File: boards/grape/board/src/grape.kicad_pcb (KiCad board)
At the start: 4 copper layers, 84 x 64 mm, 136 parts, among them J1 USB-C USB2 Device, J2 GPIO 0-27, J3 GPIO 28-55, J4 JTAG, Q1 BSS138, SW1 IMAGE[1:0], SW2 COLD RESET, SW3 PROGRAM, U1 XC7A35T-1FTG256C, U2 TPS62A02DRL, U3 TPS62A02DRL, U4 TPS62A02DRL, U5 W25Q128JVSIQ, U6 USBLC6-2SC6, U7 TPS22917DBV, X1 ASE-48.000MHz

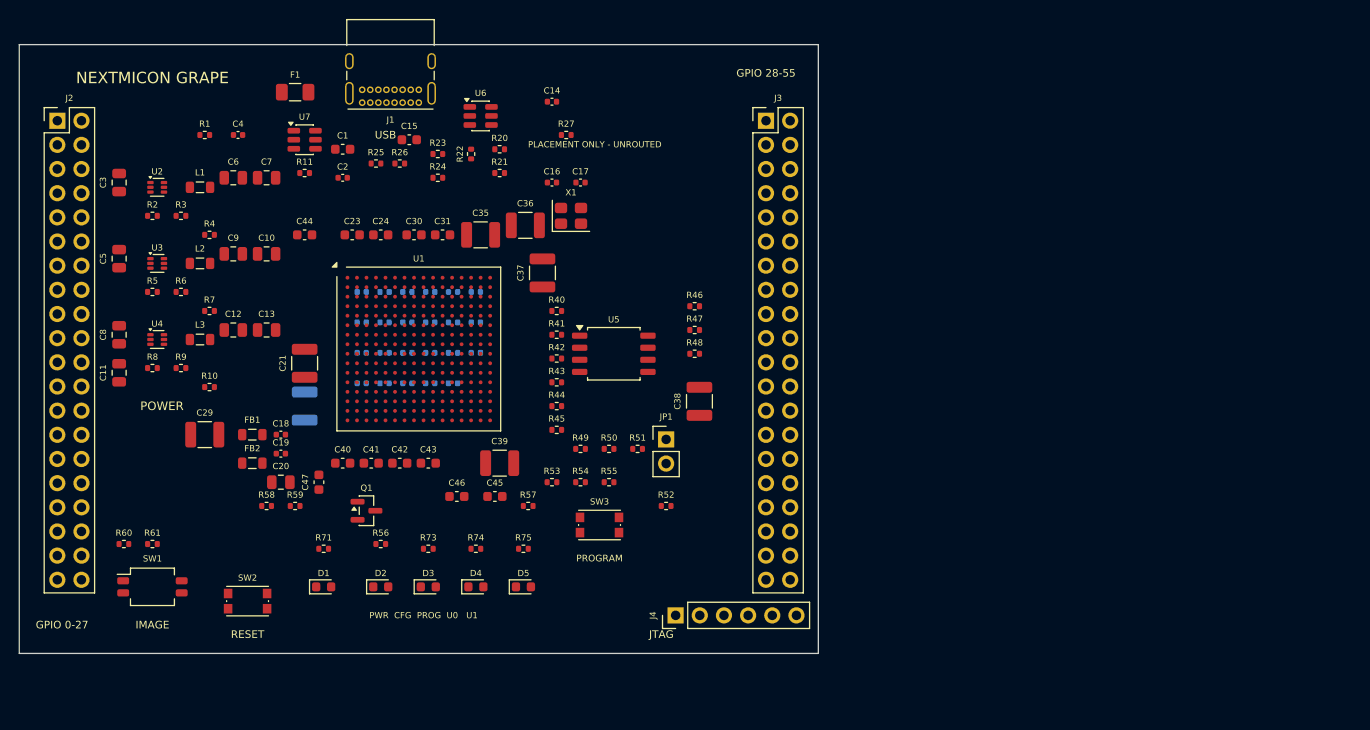
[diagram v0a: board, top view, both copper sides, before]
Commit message: wip
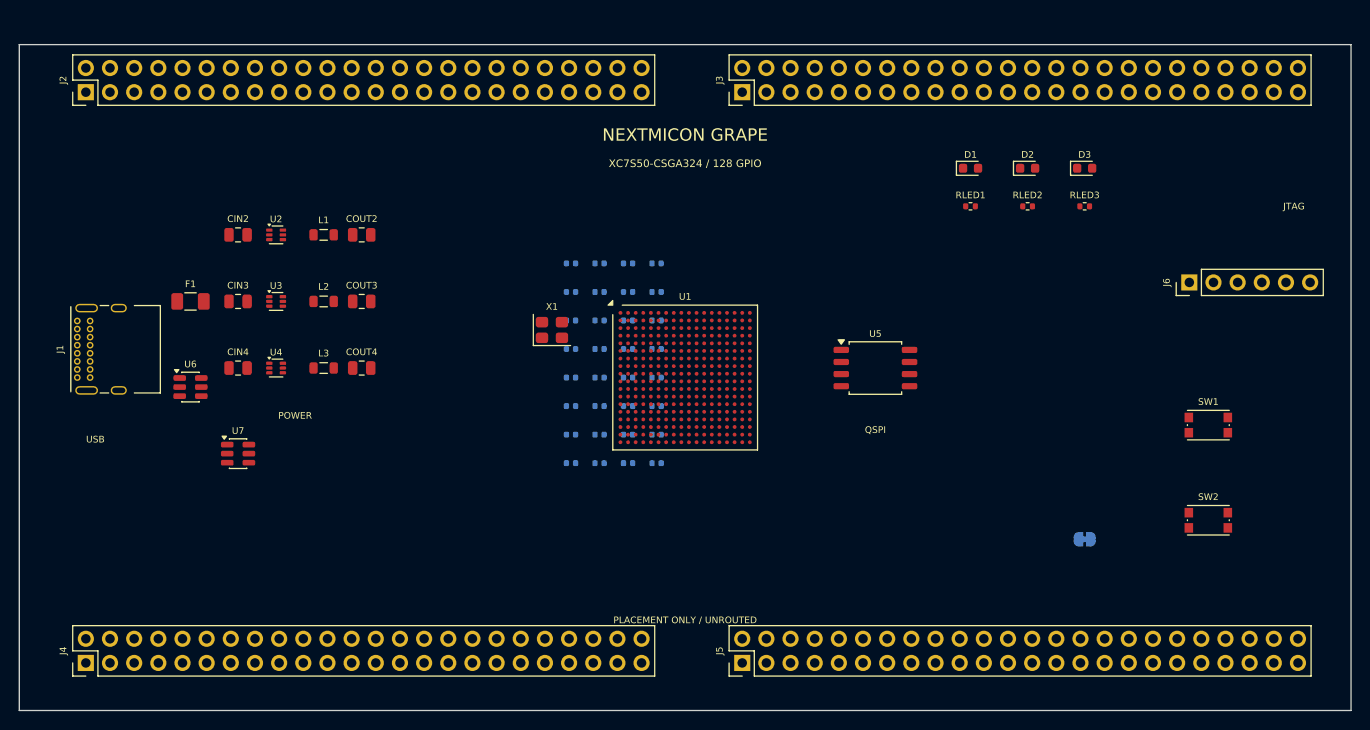
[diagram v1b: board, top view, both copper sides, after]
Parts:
- removed C1, C15: 1uF, Capacitor_SMD:C_0603_1608Metric
- removed C10, C12, C13, C6, C7, C9: 22uF, Capacitor_SMD:C_0805_2012Metric
- removed C11, C3, C5, C8: 10uF, Capacitor_SMD:C_0805_2012Metric
- removed C14: 4.7nF, Capacitor_SMD:C_0402_1005Metric
- removed C16, C17, C18, C4: 100nF, Capacitor_SMD:C_0402_1005Metric
- removed C19: 470nF, Capacitor_SMD:C_0402_1005Metric
- removed C2: 4.7nF TUNE, Capacitor_SMD:C_0402_1005Metric
- removed C52, C53, C54, C55, C56, C57, C58, C59, C60, C61, C62, C63: 0.47uF, Capacitor_SMD:C_0402_1005Metric
- removed D4: 4 LED, LED_SMD:LED_0603_1608Metric
- removed D5: 5 LED, LED_SMD:LED_0603_1608Metric
- removed FB1, FB2: 600R@100MHz, Inductor_SMD:L_0805_2012Metric
- removed Q1: BSS138, Package_TO_SOT_SMD:SOT-23
- removed R1, R10, R4, R7: 100k, Resistor_SMD:R_0402_1005Metric
- removed R11, R49, R53, R54, R55, R56, R71, R73, R74, R75: 1k, Resistor_SMD:R_0402_1005Metric
- removed R2: 66.5k 1%, Resistor_SMD:R_0402_1005Metric
- removed R20, R21, R40, R41, R42, R43, R44, R45: 22R TUNE, Resistor_SMD:R_0402_1005Metric
- removed R22: 1.5k, Resistor_SMD:R_0402_1005Metric
- removed R23, R24: 5.1k, Resistor_SMD:R_0402_1005Metric
- removed R25: 82k, Resistor_SMD:R_0402_1005Metric
- removed R26: 68k, Resistor_SMD:R_0402_1005Metric
- removed R27: 1M, Resistor_SMD:R_0402_1005Metric
- removed R3, R5, R8: 100k 1%, Resistor_SMD:R_0402_1005Metric
- removed R46: 2.4k, Resistor_SMD:R_0402_1005Metric
- removed R47, R48, R50, R51, R52: 4.7k, Resistor_SMD:R_0402_1005Metric
- removed R57, R58, R59: 0R, Resistor_SMD:R_0402_1005Metric
- removed R6: 49.9k 1%, Resistor_SMD:R_0402_1005Metric
- removed R60, R61: 10k, Resistor_SMD:R_0402_1005Metric
- removed R9: 22.1k 1%, Resistor_SMD:R_0402_1005Metric
- removed SW3: PROGRAM, Button_Switch_SMD:SW_Push_1P1T_NO_CK_KMR2
- added CIN2: 10uF, Capacitor_SMD:C_0805_2012Metric, F.Cu at (43.0, 40.0)
- added CIN3: 10uF, Capacitor_SMD:C_0805_2012Metric, F.Cu at (43.0, 47.0)
- added CIN4: 10uF, Capacitor_SMD:C_0805_2012Metric, F.Cu at (43.0, 54.0)
- added COUT2: 22uF, Capacitor_SMD:C_0805_2012Metric, F.Cu at (56.0, 40.0)
- added COUT3: 22uF, Capacitor_SMD:C_0805_2012Metric, F.Cu at (56.0, 47.0)
- added COUT4: 22uF, Capacitor_SMD:C_0805_2012Metric, F.Cu at (56.0, 54.0)
- added J5: GPIO 97-128, Connector_PinHeader_2.54mm:PinHeader_2x24_P2.54mm_Vertical, F.Cu at (96.0, 85.0)
- added J6: JTAG, Connector_PinHeader_2.54mm:PinHeader_1x06_P2.54mm_Vertical, F.Cu at (143.0, 45.0)
- added RLED1: 1k, Resistor_SMD:R_0402_1005Metric, F.Cu at (120.0, 37.0)
- added RLED2: 1k, Resistor_SMD:R_0402_1005Metric, F.Cu at (126.0, 37.0)
- added RLED3: 1k, Resistor_SMD:R_0402_1005Metric, F.Cu at (132.0, 37.0)
- C20: value 10uF -> 0.47uF; footprint Capacitor_SMD:C_0805_2012Metric -> Capacitor_SMD:C_0402_1005Metric; moved to B.Cu
- C21: value 100uF -> 0.47uF; footprint Capacitor_SMD:C_1210_3225Metric -> Capacitor_SMD:C_0402_1005Metric; moved to B.Cu
- C22: value 47uF -> 0.47uF; footprint Capacitor_SMD:C_1210_3225Metric -> Capacitor_SMD:C_0402_1005Metric
- C23, C24, C30, C31, C40, C41, C42, C43, C44, C45, C46, C47: value 4.7uF -> 0.47uF; footprint Capacitor_SMD:C_0603_1608Metric -> Capacitor_SMD:C_0402_1005Metric; moved to B.Cu
- C29, C35, C36, C37, C38, C39: value 47uF -> 0.47uF; footprint Capacitor_SMD:C_1210_3225Metric -> Capacitor_SMD:C_0402_1005Metric; moved to B.Cu
- D1: value 1 LED -> STATUS LED
- D2: value CFG DONE -> STATUS LED
- D3: value 3 LED -> STATUS LED
- F1: value 1.1A hold -> 1.1A HOLD
- J2: value GPIO 0-27 -> GPIO 1-32; footprint Connector_PinHeader_2.54mm:PinHeader_2x20_P2.54mm_Vertical -> Connector_PinHeader_2.54mm:PinHeader_2x24_P2.54mm_Vertical
- J3: value GPIO 28-55 -> GPIO 33-64; footprint Connector_PinHeader_2.54mm:PinHeader_2x20_P2.54mm_Vertical -> Connector_PinHeader_2.54mm:PinHeader_2x24_P2.54mm_Vertical
- J4: value JTAG -> GPIO 65-96; footprint Connector_PinHeader_2.54mm:PinHeader_1x06_P2.54mm_Vertical -> Connector_PinHeader_2.54mm:PinHeader_2x24_P2.54mm_Vertical
- JP1: value GOLDEN_LOCK (fit for x1) -> DEFAULT_USER; footprint Connector_PinHeader_2.54mm:PinHeader_1x02_P2.54mm_Vertical -> Jumper:SolderJumper-2_P1.3mm_Bridged_RoundedPad1.0x1.5mm; moved to B.Cu
- L1, L2, L3: value 1uH >=2.5A -> 1uH
- SW1: value IMAGE[1:0] -> PROGRAM; footprint Button_Switch_SMD:SW_DIP_SPSTx02_Slide_Omron_A6H-2101_W6.15mm_P1.27mm -> Button_Switch_SMD:SW_Push_1P1T_NO_CK_KMR2
- SW2: value COLD RESET -> USER
- U1: value XC7A35T-1FTG256C -> XC7S50-1CSGA324C; footprint Package_BGA:Xilinx_FTG256 -> Package_BGA:Xilinx_CSGA324
- X1: value ASE-48.000MHz -> 100MHz XO
- moved SW1 112.3 mm to (145.0, 60.0)
- moved SW2 101.4 mm to (145.0, 70.0)
- moved D3 81.8 mm to (132.0, 33.0)
- moved D1 81.0 mm to (120.0, 33.0)
- moved D2 81.0 mm to (126.0, 33.0)
- moved J4 62.2 mm to (27.0, 85.0)
- moved J1 46.1 mm to (26.1, 55.0), turned to 90 degrees
- moved JP1 45.2 mm to (132.0, 72.0)
- moved C29 43.2 mm to (81.0, 49.0)
- moved U6 41.7 mm to (38.0, 56.0)
- moved C20 38.2 mm to (78.0, 43.0)
- moved C22 37.2 mm to (84.0, 43.0), turned to 0 degrees
- moved C47 35.9 mm to (87.0, 61.0), turned to 0 degrees
- moved C44 35.0 mm to (78.0, 61.0)
- moved U7 33.7 mm to (43.0, 63.0)
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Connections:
- C20 pad 1: /+1V8A -> (no net)
- C20 pad 2: /AGND -> (no net)
- C21 pad 1: /+1V0 -> (no net)
- C21 pad 2: /GND -> (no net)
- C22 pad 1: /+1V0 -> (no net)
- C22 pad 2: /GND -> (no net)
- C23 pad 1: /+1V0 -> (no net)
- C23 pad 2: /GND -> (no net)
- C24 pad 1: /+1V0 -> (no net)
- C24 pad 2: /GND -> (no net)
- C25 pad 1: /+1V0 -> (no net)
- C25 pad 2: /GND -> (no net)
- C26 pad 1: /+1V0 -> (no net)
- C26 pad 2: /GND -> (no net)
- C27 pad 1: /+1V0 -> (no net)
- C27 pad 2: /GND -> (no net)
- C28 pad 1: /+1V0 -> (no net)
- C28 pad 2: /GND -> (no net)
- C29 pad 1: /+1V8 -> (no net)
- C29 pad 2: /GND -> (no net)
- C30 pad 1: /+1V8 -> (no net)
- C30 pad 2: /GND -> (no net)
- C31 pad 1: /+1V8 -> (no net)
- C31 pad 2: /GND -> (no net)
- C32 pad 1: /+1V8 -> (no net)
- C32 pad 2: /GND -> (no net)
- C33 pad 1: /+1V8 -> (no net)
- C33 pad 2: /GND -> (no net)
- C34 pad 1: /+1V8 -> (no net)
- C34 pad 2: /GND -> (no net)
- C35 pad 1: /+3V3 -> (no net)
- C35 pad 2: /GND -> (no net)
- C36 pad 1: /+3V3 -> (no net)
- C36 pad 2: /GND -> (no net)
- C37 pad 1: /+3V3 -> (no net)
- C37 pad 2: /GND -> (no net)
- C38 pad 1: /+3V3 -> (no net)
- C38 pad 2: /GND -> (no net)
- C39 pad 1: /+3V3 -> (no net)
- C39 pad 2: /GND -> (no net)
- C40 pad 1: /+3V3 -> (no net)
- C40 pad 2: /GND -> (no net)
- C41 pad 1: /+3V3 -> (no net)
- C41 pad 2: /GND -> (no net)
- C42 pad 1: /+3V3 -> (no net)
- C42 pad 2: /GND -> (no net)
- C43 pad 1: /+3V3 -> (no net)
- C43 pad 2: /GND -> (no net)
- C44 pad 1: /+3V3 -> (no net)
- C44 pad 2: /GND -> (no net)
- C45 pad 1: /+3V3 -> (no net)
- C45 pad 2: /GND -> (no net)
- C46 pad 1: /+3V3 -> (no net)
- C46 pad 2: /GND -> (no net)
- C47 pad 1: /+3V3 -> (no net)
- C47 pad 2: /GND -> (no net)
- C48 pad 1: /+3V3 -> (no net)
- C48 pad 2: /GND -> (no net)
- C49 pad 1: /+3V3 -> (no net)
- C49 pad 2: /GND -> (no net)
- C50 pad 1: /+3V3 -> (no net)
- C50 pad 2: /GND -> (no net)
- C51 pad 1: /+3V3 -> (no net)
- C51 pad 2: /GND -> (no net)
- D1 pad 1: /GND -> (no net)
- D1 pad 2: /D1_A -> (no net)
- D2 pad 1: /DONE_LED_K -> (no net)
- D2 pad 2: /DONE_LED_A -> (no net)
- D3 pad 1: /GND -> (no net)
- D3 pad 2: /D3_A -> (no net)
- F1 pad 1: /VBUS -> (no net)
- F1 pad 2: /VBUS_FUSED -> (no net)
- J1 pad A1: /GND -> (no net)
- J1 pad A12: /GND -> (no net)
- J1 pad A4: /VBUS -> (no net)
- J1 pad A5: /USB_CC1 -> (no net)
- J1 pad A6: /USB_DP_CONN -> (no net)
- J1 pad A7: /USB_DM_CONN -> (no net)
- J1 pad A8: unconnected-(J1-SBU1-PadA8) -> (no net)
- J1 pad A9: /VBUS -> (no net)
- J1 pad B1: /GND -> (no net)
- J1 pad B12: /GND -> (no net)
- J1 pad B4: /VBUS -> (no net)
- J1 pad B5: /USB_CC2 -> (no net)
- J1 pad B6: /USB_DP_CONN -> (no net)
- J1 pad B7: /USB_DM_CONN -> (no net)
- J1 pad B8: unconnected-(J1-SBU2-PadB8) -> (no net)
- J1 pad B9: /VBUS -> (no net)
- J1 pad SH: /USB_SHIELD -> (no net)
- J2 pad 1: /+3V3 -> (no net)
- J2 pad 10: /GPIO_07 -> (no net)
- J2 pad 11: /GND -> (no net)
- J2 pad 12: /GND -> (no net)
- J2 pad 13: /GPIO_08 -> (no net)
- J2 pad 14: /GPIO_09 -> (no net)
- J2 pad 15: /GPIO_10 -> (no net)
- J2 pad 16: /GPIO_11 -> (no net)
- J2 pad 17: /GPIO_12 -> (no net)
- J2 pad 18: /GPIO_13 -> (no net)
- J2 pad 19: /GPIO_14 -> (no net)
- J2 pad 2: /+5V -> (no net)
- J2 pad 20: /GPIO_15 -> (no net)
- J2 pad 21: /+3V3 -> (no net)
- J2 pad 22: /GND -> (no net)
- J2 pad 23: /GPIO_16 -> (no net)
- J2 pad 24: /GPIO_17 -> (no net)
- J2 pad 25: /GPIO_18 -> (no net)
- J2 pad 26: /GPIO_19 -> (no net)
- J2 pad 27: /GPIO_20 -> (no net)
- J2 pad 28: /GPIO_21 -> (no net)
- J2 pad 29: /GPIO_22 -> (no net)
- J2 pad 3: /GPIO_00 -> (no net)
- J2 pad 30: /GPIO_23 -> (no net)
- J2 pad 31: /GND -> (no net)
- J2 pad 32: /GND -> (no net)
- J2 pad 33: /GPIO_24 -> (no net)
- J2 pad 34: /GPIO_25 -> (no net)
- J2 pad 35: /GPIO_26 -> (no net)
- J2 pad 36: /GPIO_27 -> (no net)
- J2 pad 37: /GND -> (no net)
- J2 pad 38: /GND -> (no net)
- J2 pad 39: /+3V3 -> (no net)
- J2 pad 4: /GPIO_01 -> (no net)
- J2 pad 40: /+5V -> (no net)
- J2 pad 5: /GPIO_02 -> (no net)
- J2 pad 6: /GPIO_03 -> (no net)
- J2 pad 7: /GPIO_04 -> (no net)
- J2 pad 8: /GPIO_05 -> (no net)
- J2 pad 9: /GPIO_06 -> (no net)
- J3 pad 1: /+3V3 -> (no net)
- J3 pad 10: /GPIO_35 -> (no net)
- J3 pad 11: /GND -> (no net)
- J3 pad 12: /GND -> (no net)
- J3 pad 13: /GPIO_36 -> (no net)
- J3 pad 14: /GPIO_37 -> (no net)
- J3 pad 15: /GPIO_38 -> (no net)
- J3 pad 16: /GPIO_39 -> (no net)
- J3 pad 17: /GPIO_40 -> (no net)
- J3 pad 18: /GPIO_41 -> (no net)
- J3 pad 19: /GPIO_42 -> (no net)
- J3 pad 2: /+5V -> (no net)
- J3 pad 20: /GPIO_43 -> (no net)
- J3 pad 21: /+3V3 -> (no net)
- J3 pad 22: /GND -> (no net)
- J3 pad 23: /GPIO_44 -> (no net)
- J3 pad 24: /GPIO_45 -> (no net)
- J3 pad 25: /GPIO_46 -> (no net)
- J3 pad 26: /GPIO_47 -> (no net)
- J3 pad 27: /GPIO_48 -> (no net)
- J3 pad 28: /GPIO_49 -> (no net)
- J3 pad 29: /GPIO_50 -> (no net)
- J3 pad 3: /GPIO_28 -> (no net)
- J3 pad 30: /GPIO_51 -> (no net)
- J3 pad 31: /GND -> (no net)
- J3 pad 32: /GND -> (no net)
- J3 pad 33: /GPIO_52 -> (no net)
- J3 pad 34: /GPIO_53 -> (no net)
- J3 pad 35: /GPIO_54 -> (no net)
- J3 pad 36: /GPIO_55 -> (no net)
- J3 pad 37: /GND -> (no net)
- J3 pad 38: /GND -> (no net)
- J3 pad 39: /+3V3 -> (no net)
- J3 pad 4: /GPIO_29 -> (no net)
- J3 pad 40: /+5V -> (no net)
- J3 pad 5: /GPIO_30 -> (no net)
- J3 pad 6: /GPIO_31 -> (no net)
- J3 pad 7: /GPIO_32 -> (no net)
- J3 pad 8: /GPIO_33 -> (no net)
- J3 pad 9: /GPIO_34 -> (no net)
- J4 pad 1: /+3V3 -> (no net)
- J4 pad 2: /GND -> (no net)
- J4 pad 3: /JTAG_TCK -> (no net)
- J4 pad 4: /JTAG_TMS -> (no net)
- J4 pad 5: /JTAG_TDI -> (no net)
- J4 pad 6: /JTAG_TDO -> (no net)
- JP1 pad 1: /QSPI_IO2 -> (no net)
- JP1 pad 2: /GND -> (no net)
- L1 pad 1: /+1V0_SW -> (no net)
- L1 pad 2: /+1V0 -> (no net)
- L2 pad 1: /+1V8_SW -> (no net)
- L2 pad 2: /+1V8 -> (no net)
- L3 pad 1: /+3V3_SW -> (no net)
- L3 pad 2: /+3V3 -> (no net)
- SW1 pad 1: /IMAGE0 -> (no net)
- SW1 pad 2: /IMAGE1 -> (no net)
- SW2 pad 1: /PWR_EN -> (no net)
- SW2 pad 2: /GND -> (no net)
- U1 pad A1: /GND -> (no net)
- U1 pad A10: unconnected-(U1A-IO_L3N_T0_DQS_AD1N_15-PadA10) -> (no net)
- U1 pad A11: /GND -> (no net)
- U1 pad A12: unconnected-(U1A-IO_L5N_T0_AD9N_15-PadA12) -> (no net)
- U1 pad A13: unconnected-(U1A-IO_L7P_T1_AD2P_15-PadA13) -> (no net)
- U1 pad A14: unconnected-(U1A-IO_L7N_T1_AD2N_15-PadA14) -> (no net)
- U1 pad A15: unconnected-(U1A-IO_L9N_T1_DQS_AD3N_15-PadA15) -> (no net)
- U1 pad A16: /+3V3 -> (no net)
- U1 pad A2: /USER_LED1 -> (no net)
- U1 pad A3: /IMAGE0 -> (no net)
- U1 pad A4: /PROG_LED -> (no net)
- U1 pad A5: /USER_LED0 -> (no net)
- U1 pad A6: /+3V3 -> (no net)
- U1 pad A7: /VBUS_SENSE -> (no net)
- U1 pad A8: unconnected-(U1A-IO_L2P_T0_AD8P_15-PadA8) -> (no net)
- U1 pad A9: unconnected-(U1A-IO_L2N_T0_AD8N_15-PadA9) -> (no net)
- U1 pad B1: /GPIO_00 -> (no net)
- U1 pad B10: unconnected-(U1A-IO_L4P_T0_15-PadB10) -> (no net)
- U1 pad B11: unconnected-(U1A-IO_L4N_T0_15-PadB11) -> (no net)
- U1 pad B12: unconnected-(U1A-IO_L5P_T0_AD9P_15-PadB12) -> (no net)
- U1 pad B13: /+3V3 -> (no net)
- U1 pad B14: unconnected-(U1A-IO_L8N_T1_AD10N_15-PadB14) -> (no net)
- U1 pad B15: unconnected-(U1A-IO_L9P_T1_DQS_AD3P_15-PadB15) -> (no net)
- U1 pad B16: unconnected-(U1A-IO_L10N_T1_AD11N_15-PadB16) -> (no net)
- U1 pad B2: /GPIO_01 -> (no net)
- U1 pad B3: /+3V3 -> (no net)
- U1 pad B4: /IMAGE1 -> (no net)
- U1 pad B5: /USB_DM -> (no net)
- U1 pad B6: /USB_DP -> (no net)
- U1 pad B7: /USB_PULLUP -> (no net)
- U1 pad B8: /GND -> (no net)
- U1 pad B9: unconnected-(U1A-IO_L3P_T0_DQS_AD1P_15-PadB9) -> (no net)
- U1 pad C1: /GPIO_02 -> (no net)
- U1 pad C10: /+3V3 -> (no net)
- U1 pad C11: unconnected-(U1A-IO_L11P_T1_SRCC_15-PadC11) -> (no net)
- U1 pad C12: unconnected-(U1A-IO_L11N_T1_SRCC_15-PadC12) -> (no net)
- U1 pad C13: unconnected-(U1A-IO_L12N_T1_MRCC_15-PadC13) -> (no net)
- U1 pad C14: unconnected-(U1A-IO_L8P_T1_AD10P_15-PadC14) -> (no net)
- U1 pad C15: /GND -> (no net)
- U1 pad C16: unconnected-(U1A-IO_L10P_T1_AD11P_15-PadC16) -> (no net)
- U1 pad C2: /GPIO_03 -> (no net)
- U1 pad C3: /GPIO_04 -> (no net)
- U1 pad C4: /GPIO_05 -> (no net)
- U1 pad C5: /GND -> (no net)
- U1 pad C6: /GPIO_06 -> (no net)
- U1 pad C7: /GPIO_07 -> (no net)
- U1 pad C8: unconnected-(U1A-IO_L1P_T0_AD0P_15-PadC8) -> (no net)
- U1 pad C9: unconnected-(U1A-IO_L1N_T0_AD0N_15-PadC9) -> (no net)
- U1 pad D1: /GPIO_08 -> (no net)
- U1 pad D10: unconnected-(U1A-IO_0_15-PadD10) -> (no net)
- U1 pad D11: unconnected-(U1A-IO_L14N_T2_SRCC_15-PadD11) -> (no net)
- U1 pad D12: /GND -> (no net)
- U1 pad D13: unconnected-(U1A-IO_L12P_T1_MRCC_15-PadD13) -> (no net)
- U1 pad D14: unconnected-(U1A-IO_L15P_T2_DQS_15-PadD14) -> (no net)
- U1 pad D15: unconnected-(U1A-IO_L15N_T2_DQS_ADV_B_15-PadD15) -> (no net)
- U1 pad D16: unconnected-(U1A-IO_L17N_T2_A25_15-PadD16) -> (no net)
- U1 pad D2: /GND -> (no net)
- U1 pad D3: /GPIO_09 -> (no net)
- U1 pad D4: /GPIO_10 -> (no net)
- U1 pad D5: /GPIO_11 -> (no net)
- U1 pad D6: /GPIO_12 -> (no net)
- U1 pad D7: /+3V3 -> (no net)
- U1 pad D8: unconnected-(U1A-IO_L6P_T0_15-PadD8) -> (no net)
- U1 pad D9: unconnected-(U1A-IO_L6N_T0_VREF_15-PadD9) -> (no net)
- U1 pad E1: /GPIO_13 -> (no net)
- U1 pad E10: /+1V0 -> (no net)
- U1 pad E11: unconnected-(U1A-IO_L14P_T2_SRCC_15-PadE11) -> (no net)
- U1 pad E12: unconnected-(U1A-IO_L13P_T2_MRCC_15-PadE12) -> (no net)
- U1 pad E13: unconnected-(U1A-IO_L13N_T2_MRCC_15-PadE13) -> (no net)
- U1 pad E14: /+3V3 -> (no net)
- U1 pad E15: unconnected-(U1A-IO_L18N_T2_A23_15-PadE15) -> (no net)
- U1 pad E16: unconnected-(U1A-IO_L17P_T2_A26_15-PadE16) -> (no net)
- U1 pad E2: /GPIO_14 -> (no net)
- U1 pad E3: /CLK48 -> (no net)
- U1 pad E4: /+3V3 -> (no net)
- U1 pad E5: /GPIO_15 -> (no net)
- U1 pad E6: /GPIO_16 -> (no net)
- U1 pad E7: /CFGBVS_3V3 -> (no net)
- U1 pad E8: /QSPI_CCLK_FPGA -> (no net)
- U1 pad E9: /GND -> (no net)
- U1 pad F1: /+3V3 -> (no net)
- U1 pad F10: /GND -> (no net)
- U1 pad F11: /+1V0 -> (no net)
- U1 pad F12: unconnected-(U1A-IO_L16P_T2_A28_15-PadF12) -> (no net)
- U1 pad F13: unconnected-(U1A-IO_L16N_T2_A27_15-PadF13) -> (no net)
- U1 pad F14: unconnected-(U1A-IO_L21N_T3_DQS_A18_15-PadF14) -> (no net)
- U1 pad F15: unconnected-(U1A-IO_L18P_T2_A24_15-PadF15) -> (no net)
- U1 pad F16: /GND -> (no net)
- U1 pad F2: /GPIO_17 -> (no net)
- U1 pad F3: /GPIO_18 -> (no net)
- U1 pad F4: /GPIO_19 -> (no net)
- U1 pad F5: /GPIO_20 -> (no net)
- U1 pad F6: /GND -> (no net)
- U1 pad F7: /+1V0 -> (no net)
- U1 pad F8: /GND -> (no net)
- U1 pad F9: /+1V0 -> (no net)
- U1 pad G1: /GPIO_21 -> (no net)
- U1 pad G10: /+1V8 -> (no net)
- U1 pad G11: unconnected-(U1A-IO_25_15-PadG11) -> (no net)
- U1 pad G12: unconnected-(U1A-IO_L19N_T3_A21_VREF_15-PadG12) -> (no net)
- U1 pad G13: /GND -> (no net)
- U1 pad G14: unconnected-(U1A-IO_L21P_T3_DQS_15-PadG14) -> (no net)
- U1 pad G15: unconnected-(U1A-IO_L24N_T3_RS0_15-PadG15) -> (no net)
- U1 pad G16: unconnected-(U1A-IO_L22N_T3_A16_15-PadG16) -> (no net)
- U1 pad G2: /GPIO_22 -> (no net)
- U1 pad G3: /GND -> (no net)
- U1 pad G4: /GPIO_23 -> (no net)
- U1 pad G5: /GPIO_24 -> (no net)
- U1 pad G6: /+1V0 -> (no net)
- U1 pad G7: /AGND -> (no net)
- U1 pad G8: /+1V8A -> (no net)
- U1 pad G9: /GND -> (no net)
- U1 pad H1: /GPIO_25 -> (no net)
- U1 pad H10: /DONE -> (no net)
- U1 pad H11: unconnected-(U1A-IO_L19P_T3_A22_15-PadH11) -> (no net)
- U1 pad H12: unconnected-(U1A-IO_L20P_T3_A20_15-PadH12) -> (no net)
- U1 pad H13: unconnected-(U1A-IO_L20N_T3_A19_15-PadH13) -> (no net)
- U1 pad H14: unconnected-(U1A-IO_L24P_T3_RS1_15-PadH14) -> (no net)
- U1 pad H15: /+3V3 -> (no net)
- U1 pad H16: unconnected-(U1A-IO_L22P_T3_A17_15-PadH16) -> (no net)
- U1 pad H2: /GPIO_26 -> (no net)
- U1 pad H3: /GPIO_27 -> (no net)
- U1 pad H4: /GPIO_28 -> (no net)
- U1 pad H5: /GPIO_29 -> (no net)
- U1 pad H6: /GND -> (no net)
- U1 pad H7: /VREFN_AGND -> (no net)
- U1 pad H8: unconnected-(U1C-VP_0-PadH8) -> (no net)
- U1 pad H9: /+1V0 -> (no net)
- U1 pad J1: /GPIO_30 -> (no net)
- U1 pad J10: /+1V8 -> (no net)
- U1 pad J11: /GND -> (no net)
- U1 pad J12: /+3V3 -> (no net)
- U1 pad J13: /QSPI_IO0_FPGA -> (no net)
- U1 pad J14: /QSPI_IO1_FPGA -> (no net)
- U1 pad J15: unconnected-(U1A-IO_L23P_T3_FOE_B_15-PadJ15) -> (no net)
- U1 pad J16: unconnected-(U1A-IO_L23N_T3_FWE_B_15-PadJ16) -> (no net)
- U1 pad J2: /+3V3 -> (no net)
- U1 pad J3: /GPIO_31 -> (no net)
- U1 pad J4: /GPIO_32 -> (no net)
- U1 pad J5: /GPIO_33 -> (no net)
- U1 pad J6: /+1V0 -> (no net)
- U1 pad J7: unconnected-(U1C-VN_0-PadJ7) -> (no net)
- U1 pad J8: /VREFP_AGND -> (no net)
- U1 pad J9: /GND -> (no net)
- U1 pad K1: /GPIO_34 -> (no net)
- U1 pad K10: /INIT_B -> (no net)
- U1 pad K11: /+1V8 -> (no net)
- U1 pad K12: unconnected-(U1A-IO_0_14-PadK12) -> (no net)
- U1 pad K13: unconnected-(U1A-IO_L5P_T0_D06_14-PadK13) -> (no net)
- U1 pad K14: /GND -> (no net)
- U1 pad K15: /QSPI_IO2_FPGA -> (no net)
- U1 pad K16: /QSPI_IO3_FPGA -> (no net)
- U1 pad K2: /GPIO_35 -> (no net)
- U1 pad K3: /GPIO_36 -> (no net)
- U1 pad K4: /GND -> (no net)
- U1 pad K5: /GPIO_37 -> (no net)
- U1 pad K6: /GND -> (no net)
- U1 pad K7: unconnected-(U1C-DXN_0-PadK7) -> (no net)
- U1 pad K8: unconnected-(U1C-DXP_0-PadK8) -> (no net)
- U1 pad K9: /+1V0 -> (no net)
- U1 pad L1: /GND -> (no net)
- U1 pad L10: /+1V8 -> (no net)
- U1 pad L11: /GND -> (no net)
- U1 pad L12: /QSPI_CS_B_FPGA -> (no net)
- U1 pad L13: unconnected-(U1A-IO_L5N_T0_D07_14-PadL13) -> (no net)
- U1 pad L14: unconnected-(U1A-IO_L4P_T0_D04_14-PadL14) -> (no net)
- U1 pad L15: /PUDC_B -> (no net)
- U1 pad L16: /+3V3 -> (no net)
- U1 pad L2: /GPIO_38 -> (no net)
- U1 pad L3: /GPIO_39 -> (no net)
- U1 pad L4: /GPIO_40 -> (no net)
- U1 pad L5: /GPIO_41 -> (no net)
- U1 pad L6: /+3V3 -> (no net)
- U1 pad L7: /JTAG_TCK -> (no net)
- U1 pad L8: /+1V0 -> (no net)
- U1 pad L9: /PROGRAM_B -> (no net)
- U1 pad M1: /GPIO_42 -> (no net)
- U1 pad M10: /MODE_M1 -> (no net)
- U1 pad M11: /MODE_M2 -> (no net)
- U1 pad M12: unconnected-(U1A-IO_L6N_T0_D08_VREF_14-PadM12) -> (no net)
- U1 pad M13: /+3V3 -> (no net)
- U1 pad M14: unconnected-(U1A-IO_L4N_T0_D05_14-PadM14) -> (no net)
- U1 pad M15: unconnected-(U1A-IO_L3N_T0_DQS_EMCCLK_14-PadM15) -> (no net)
- U1 pad M16: unconnected-(U1A-IO_L7P_T1_D09_14-PadM16) -> (no net)
- U1 pad M2: /GPIO_43 -> (no net)
- U1 pad M3: /+3V3 -> (no net)
- U1 pad M4: /GPIO_44 -> (no net)
- U1 pad M5: /GPIO_45 -> (no net)
- U1 pad M6: unconnected-(U1A-IO_L19P_T3_A10_D26_14-PadM6) -> (no net)
- U1 pad M7: /JTAG_TMS -> (no net)
- U1 pad M8: /GND -> (no net)
- U1 pad M9: /MODE_M0 -> (no net)
- U1 pad N1: /GPIO_46 -> (no net)
- U1 pad N10: /+3V3 -> (no net)
- U1 pad N11: unconnected-(U1A-IO_L13P_T2_MRCC_14-PadN11) -> (no net)
- U1 pad N12: unconnected-(U1A-IO_L13N_T2_MRCC_14-PadN12) -> (no net)
- U1 pad N13: unconnected-(U1A-IO_L11P_T1_SRCC_14-PadN13) -> (no net)
- U1 pad N14: unconnected-(U1A-IO_L12P_T1_MRCC_14-PadN14) -> (no net)
- U1 pad N15: /GND -> (no net)
- U1 pad N16: unconnected-(U1A-IO_L7N_T1_D10_14-PadN16) -> (no net)
- U1 pad N2: /GPIO_47 -> (no net)
- U1 pad N3: /GPIO_48 -> (no net)
- U1 pad N4: /GPIO_49 -> (no net)
- U1 pad N5: /GND -> (no net)
- U1 pad N6: unconnected-(U1A-IO_L19N_T3_A09_D25_VREF_14-PadN6) -> (no net)
- U1 pad N7: /JTAG_TDI -> (no net)
- U1 pad N8: /JTAG_TDO -> (no net)
- U1 pad N9: unconnected-(U1A-IO_L18P_T2_A12_D28_14-PadN9) -> (no net)
- U1 pad P1: /GPIO_50 -> (no net)
- U1 pad P10: unconnected-(U1A-IO_L14P_T2_SRCC_14-PadP10) -> (no net)
- U1 pad P11: unconnected-(U1A-IO_L14N_T2_SRCC_14-PadP11) -> (no net)
- U1 pad P12: /GND -> (no net)
- U1 pad P13: unconnected-(U1A-IO_L11N_T1_SRCC_14-PadP13) -> (no net)
- U1 pad P14: unconnected-(U1A-IO_L12N_T1_MRCC_14-PadP14) -> (no net)
- U1 pad P15: unconnected-(U1A-IO_L8P_T1_D11_14-PadP15) -> (no net)
- U1 pad P16: unconnected-(U1A-IO_L8N_T1_D12_14-PadP16) -> (no net)
- U1 pad P2: /GND -> (no net)
- U1 pad P3: /GPIO_51 -> (no net)
- U1 pad P4: /GPIO_52 -> (no net)
- U1 pad P5: /GPIO_53 -> (no net)
- U1 pad P6: unconnected-(U1A-IO_25_14-PadP6) -> (no net)
- U1 pad P7: /+3V3 -> (no net)
- U1 pad P8: unconnected-(U1A-IO_L20P_T3_A08_D24_14-PadP8) -> (no net)
- U1 pad P9: unconnected-(U1A-IO_L18N_T2_A11_D27_14-PadP9) -> (no net)
- U1 pad R1: /GPIO_54 -> (no net)
- U1 pad R10: unconnected-(U1A-IO_L17P_T2_A14_D30_14-PadR10) -> (no net)
- U1 pad R11: unconnected-(U1A-IO_L17N_T2_A13_D29_14-PadR11) -> (no net)
- U1 pad R12: unconnected-(U1A-IO_L15P_T2_DQS_RDWR_B_14-PadR12) -> (no net)
- U1 pad R13: unconnected-(U1A-IO_L16P_T2_CSI_B_14-PadR13) -> (no net)
- U1 pad R14: /+3V3 -> (no net)
- U1 pad R15: unconnected-(U1A-IO_L9P_T1_DQS_14-PadR15) -> (no net)
- U1 pad R16: unconnected-(U1A-IO_L9N_T1_DQS_D13_14-PadR16) -> (no net)
- U1 pad R2: /GPIO_55 -> (no net)
- U1 pad R3: unconnected-(U1B-IO_L8P_T1_34-PadR3) -> (no net)
- U1 pad R4: /+3V3 -> (no net)
- U1 pad R5: unconnected-(U1A-IO_L23P_T3_A03_D19_14-PadR5) -> (no net)
- U1 pad R6: unconnected-(U1A-IO_L24P_T3_A01_D17_14-PadR6) -> (no net)
- U1 pad R7: unconnected-(U1A-IO_L24N_T3_A00_D16_14-PadR7) -> (no net)
- U1 pad R8: unconnected-(U1A-IO_L20N_T3_A07_D23_14-PadR8) -> (no net)
- U1 pad R9: /GND -> (no net)
- U1 pad T1: /+3V3 -> (no net)
- U1 pad T10: unconnected-(U1A-IO_L22N_T3_A04_D20_14-PadT10) -> (no net)
- U1 pad T11: /+3V3 -> (no net)
- U1 pad T12: unconnected-(U1A-IO_L15N_T2_DQS_DOUT_CSO_B_14-PadT12) -> (no net)
- U1 pad T13: unconnected-(U1A-IO_L16N_T2_A15_D31_14-PadT13) -> (no net)
- U1 pad T14: unconnected-(U1A-IO_L10P_T1_D14_14-PadT14) -> (no net)
- U1 pad T15: unconnected-(U1A-IO_L10N_T1_D15_14-PadT15) -> (no net)
- U1 pad T16: /GND -> (no net)
- U1 pad T2: unconnected-(U1B-IO_L8N_T1_34-PadT2) -> (no net)
- U1 pad T3: unconnected-(U1B-IO_L9N_T1_DQS_34-PadT3) -> (no net)
- U1 pad T4: unconnected-(U1B-IO_L9P_T1_DQS_34-PadT4) -> (no net)
- U1 pad T5: unconnected-(U1A-IO_L23N_T3_A02_D18_14-PadT5) -> (no net)
- U1 pad T6: /GND -> (no net)
- U1 pad T7: unconnected-(U1A-IO_L21P_T3_DQS_14-PadT7) -> (no net)
- U1 pad T8: unconnected-(U1A-IO_L21N_T3_DQS_A06_D22_14-PadT8) -> (no net)
- U1 pad T9: unconnected-(U1A-IO_L22P_T3_A05_D21_14-PadT9) -> (no net)
- U2 pad 1: /GND -> (no net)
- U2 pad 2: /+1V0_SW -> (no net)
- U2 pad 3: /+5V -> (no net)
- U2 pad 4: /PWR_EN -> (no net)
- U2 pad 5: /+1V0_FB -> (no net)
- U2 pad 6: /EN_1V8 -> (no net)
- U3 pad 1: /GND -> (no net)
- U3 pad 2: /+1V8_SW -> (no net)
- U3 pad 3: /+5V -> (no net)
- U3 pad 4: /EN_1V8 -> (no net)
- U3 pad 5: /+1V8_FB -> (no net)
- U3 pad 6: /EN_3V3 -> (no net)
- U4 pad 1: /GND -> (no net)
- U4 pad 2: /+3V3_SW -> (no net)
- U4 pad 3: /+5V -> (no net)
- U4 pad 4: /EN_3V3 -> (no net)
- U4 pad 5: /+3V3_FB -> (no net)
- U4 pad 6: /POWER_GOOD -> (no net)
- U5 pad 1: /QSPI_CS_B -> (no net)
- U5 pad 2: /QSPI_IO1 -> (no net)
- U5 pad 3: /QSPI_IO2 -> (no net)
- U5 pad 4: /GND -> (no net)
- U5 pad 5: /QSPI_IO0 -> (no net)
- U5 pad 6: /QSPI_CCLK -> (no net)
- U5 pad 7: /QSPI_IO3 -> (no net)
- U5 pad 8: /+3V3 -> (no net)
- U6 pad 1: /USB_DP_CONN -> (no net)
- U6 pad 2: /GND -> (no net)
- U6 pad 3: /USB_DM_CONN -> (no net)
- U6 pad 4: /USB_DM_PROT -> (no net)
- U6 pad 5: /VBUS -> (no net)
- U6 pad 6: /USB_DP_PROT -> (no net)
- U7 pad 1: /VBUS_FUSED -> (no net)
- U7 pad 2: /GND -> (no net)
- U7 pad 3: /VBUS_FUSED -> (no net)
- U7 pad 4: /USB_INRUSH_CT -> (no net)
- U7 pad 5: /USB_QOD -> (no net)
- U7 pad 6: /+5V -> (no net)
- X1 pad 1: /+3V3 -> (no net)
- X1 pad 2: /GND -> (no net)
- X1 pad 3: /CLK48 -> (no net)
- X1 pad 4: /+3V3 -> (no net)
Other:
- board size 84 x 64 mm -> 140 x 70 mm
- board text added: "DEFAULT USER"
- board text added: "PLACEMENT ONLY / UNROUTED"
- board text added: "QSPI"
- board text added: "XC7S50-CSGA324 / 128 GPIO"
- board text removed: "GPIO 0-27"
- board text removed: "GPIO 28-55"
- board text removed: "IMAGE"
- board text removed: "PLACEMENT ONLY - UNROUTED"
- board text removed: "PROGRAM"
- board text removed: "PWR CFG PROG U0 U1"
- board text removed: "RESET"
